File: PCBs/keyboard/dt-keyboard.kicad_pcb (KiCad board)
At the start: 2 copper layers, 87 parts

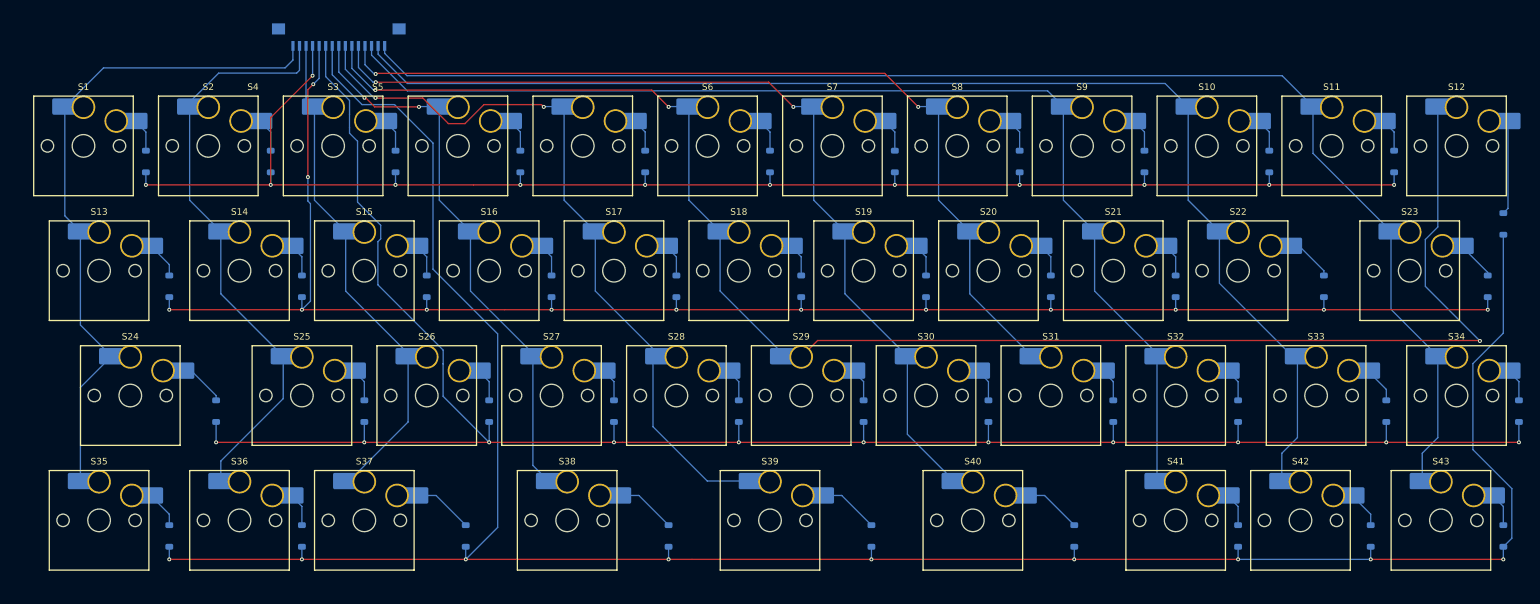
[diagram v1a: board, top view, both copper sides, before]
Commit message: Verification
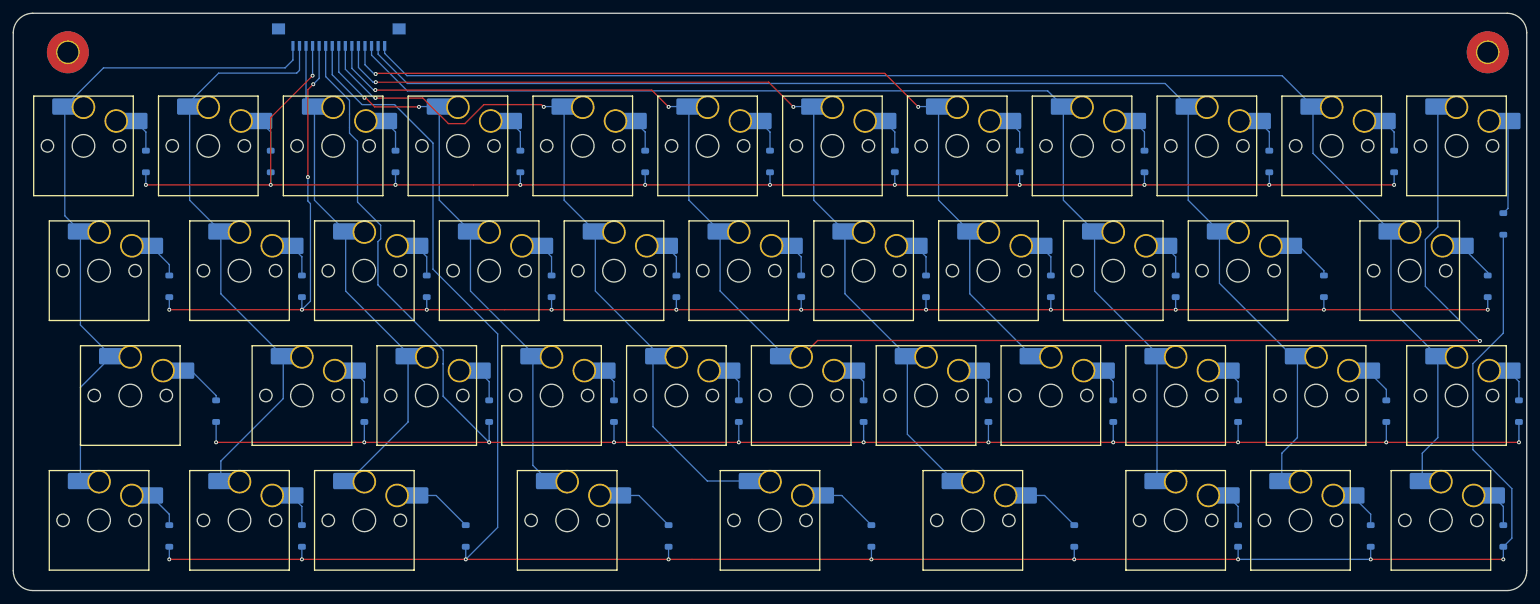
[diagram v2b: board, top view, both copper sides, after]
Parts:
- added H1: MountingHole_Pad, MountingHole:MountingHole_3.2mm_M3_Pad_TopBottom, F.Cu at (41.1, 56.2)
- added H2: MountingHole_Pad, MountingHole:MountingHole_3.2mm_M3_Pad_TopBottom, F.Cu at (257.8, 56.2)
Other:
- board outline added: 231 x 88.1 mm
